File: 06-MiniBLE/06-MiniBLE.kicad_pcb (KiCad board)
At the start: 2 copper layers, 23 parts, among them J1 Conn_01x10, U1 ICM-20602, Y1 Crystal

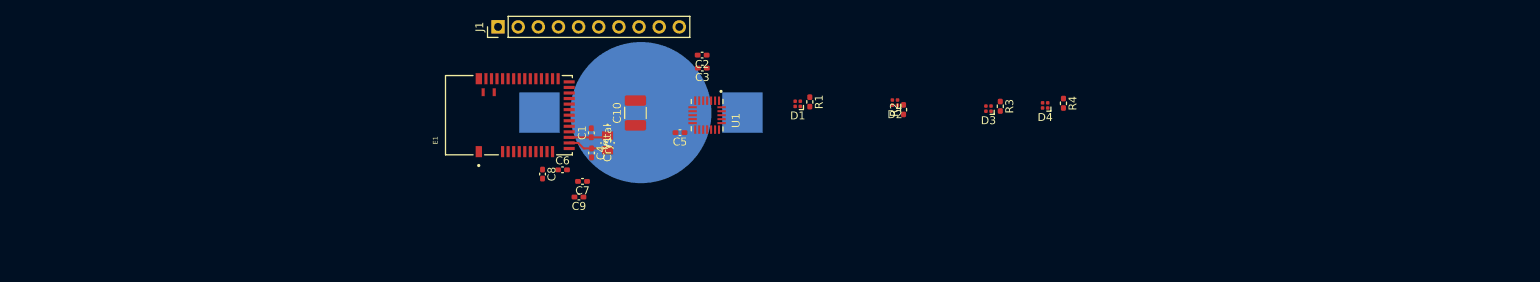
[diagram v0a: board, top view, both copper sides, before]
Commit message: Updating layout for wand
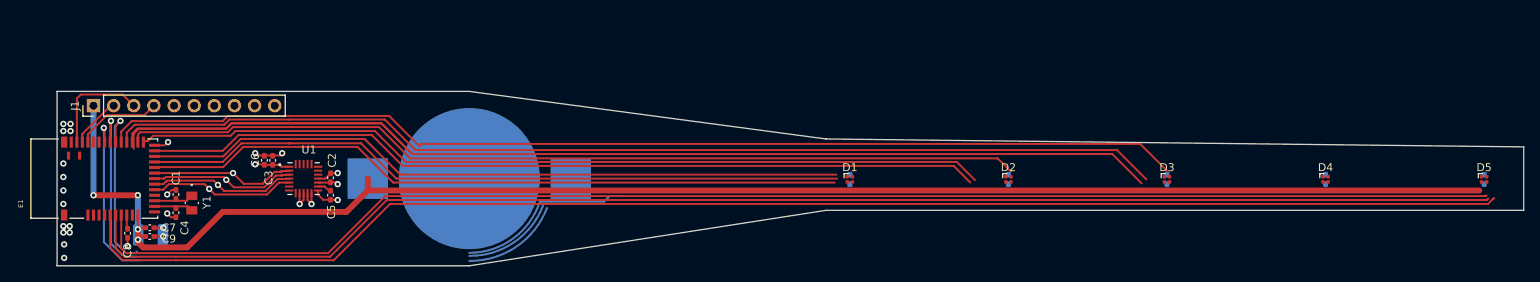
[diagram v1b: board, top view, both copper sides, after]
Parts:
- added D5: LED_ARGB, LED_SMD:LED_Lumex_SML-LX0303SIUPGUSB, F.Cu at (248.0, 93.1)
- added R5: 1k, Resistor_SMD:R_0402_1005Metric_Pad0.72x0.64mm_HandSolder, B.Cu at (248.0, 93.1)
- C10, R1, R2, R3, R4: moved to B.Cu
- moved C10 63.1 mm to (79.8, 100.1), turned to 0 degrees
- moved C3 55.4 mm to (95.2, 90.7), turned to 90 degrees
- moved C7 54.9 mm to (79.7, 99.2), turned to 0 degrees
- moved C9 54.4 mm to (79.7, 100.3), turned to 0 degrees
- moved Y1 53.0 mm to (85.0, 96.1)
- moved C1 53.0 mm to (83.0, 95.0)
- moved C4 53.0 mm to (83.0, 97.3)
- moved E1 52.9 mm to (72.7, 93.0)
- moved C8 52.9 mm to (76.9, 99.9)
- moved J1 52.0 mm to (72.6, 83.8)
- moved U1 51.5 mm to (99.1, 93.0), turned to 0 degrees
- moved C2 49.4 mm to (102.5, 92.9), turned to -90 degrees
- moved C5 44.8 mm to (102.5, 95.1), turned to -90 degrees
- moved C6 37.6 mm to (94.2, 90.7), turned to 90 degrees
- moved D4 36.6 mm to (228.0, 93.1), turned to 0 degrees
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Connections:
- net Net-(E1-Pad10) renamed no_connect_44
- net Net-(E1-Pad15) renamed no_connect_45
- net Net-(U1-Pad6) renamed no_connect_46
- net Net-(U1-Pad7) renamed no_connect_47
- net Net-(U1-Pad8) renamed no_connect_48
- E1 pad 16: /SPI_MISO -> /GYRO_CS
- E1 pad 17: /SPI_MOSI -> /SPI_MISO
- E1 pad 18: /SPI_CLK -> /SPI_MOSI
- E1 pad 19: /GYRO_CS -> /SPI_CLK
- E1 pad 2: /LED4R -> Net-(E1-Pad2)
- E1 pad 3: /LED4G -> Net-(E1-Pad3)
- E1 pad 30: Net-(E1-Pad30) -> /LED5R
- E1 pad 31: Net-(E1-Pad31) -> /LED5G
- E1 pad 32: Net-(E1-Pad32) -> /LED5B
- E1 pad 4: /LED4B -> Net-(E1-Pad4)
- E1 pad 6: Net-(E1-Pad6) -> /LED4R
- E1 pad 7: Net-(E1-Pad7) -> /LED4G
- E1 pad 8: Net-(E1-Pad8) -> /LED4B
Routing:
- net +BATT: track 0.00 -> 209.6 mm, vias 0 -> 6
- net /LED4R: track 0.00 -> 182.6 mm
- net /LED4G: track 0.00 -> 180.8 mm
- net /LED4B: track 0.00 -> 179.7 mm
- net /LED3R: track 0.00 -> 171.1 mm
- net /LED3B: track 0.00 -> 137.3 mm
- net /LED3G: track 0.00 -> 133.6 mm
- net /LED2B: track 0.00 -> 113.8 mm
- net /LED2G: track 0.00 -> 108.3 mm
- net /LED2R: track 0.00 -> 106.3 mm
- net /LED1G: track 0.00 -> 89.1 mm
- net /LED1B: track 0.00 -> 88.8 mm
- net /LED1R: track 0.00 -> 88.7 mm
- net /LED5R: track 0.00 -> 32.4 mm, vias 0 -> 1
- net GND: track 0.00 -> 23.2 mm, vias 0 -> 26
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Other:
- board outline added: 185 x 22 mm
